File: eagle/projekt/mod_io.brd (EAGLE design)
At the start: 102.5 x 80 mm, 47 parts, among them IC1 PCF8574P

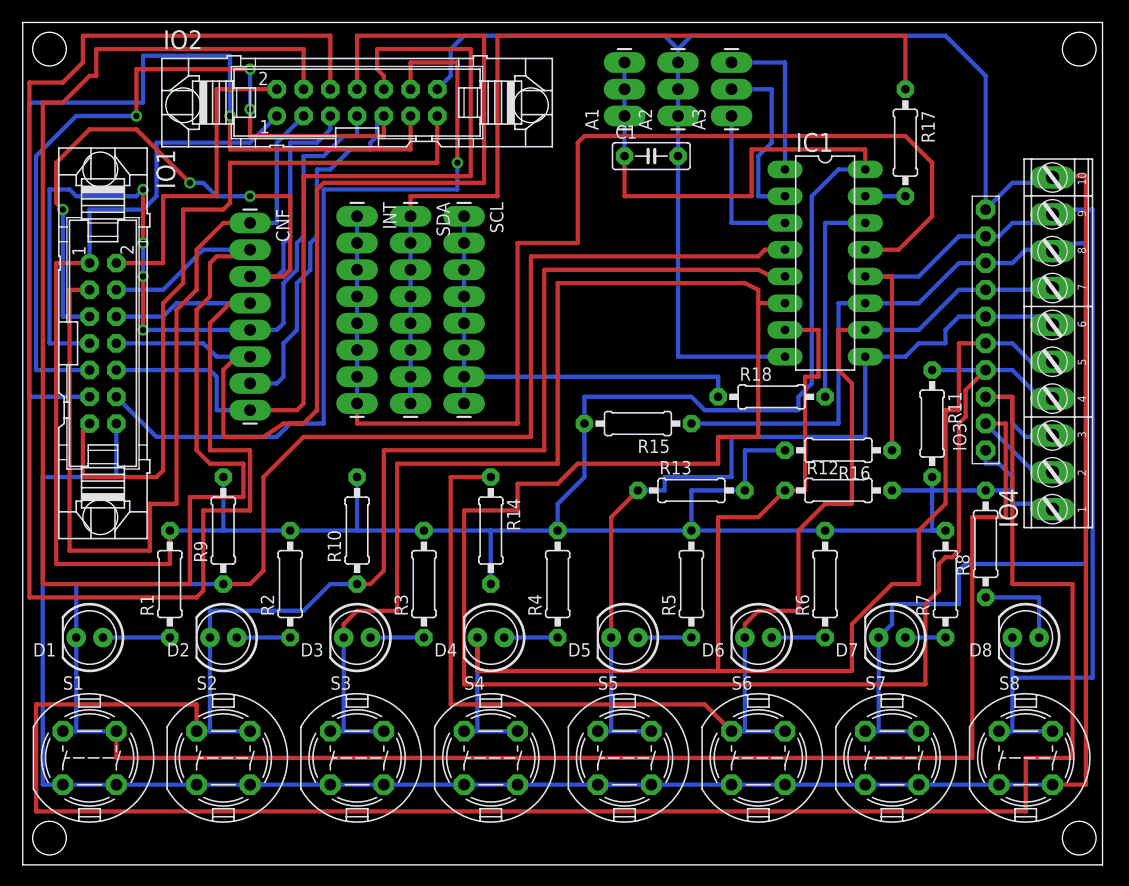
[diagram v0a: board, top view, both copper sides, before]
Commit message: Deska, modul IO
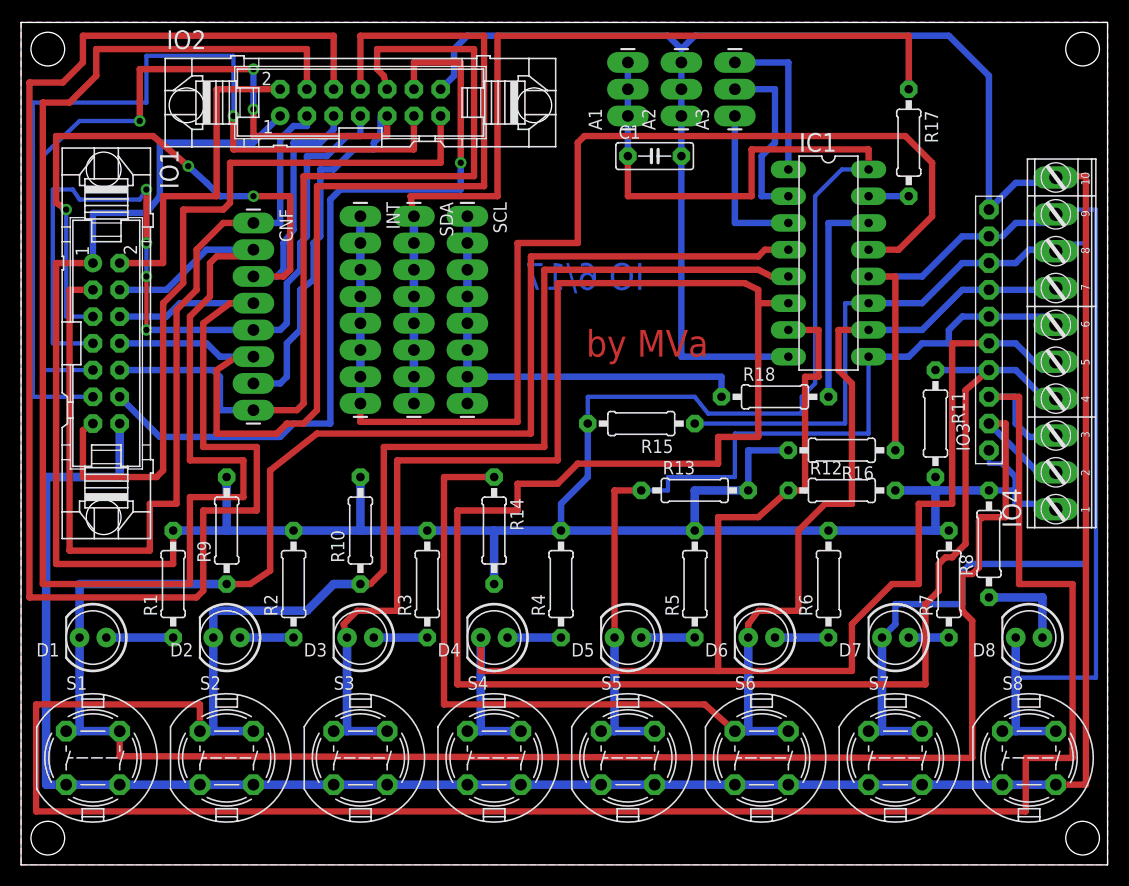
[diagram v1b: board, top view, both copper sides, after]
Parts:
- moved D6 0.32 mm to (70.2, 21.6)
- moved D7 0.32 mm to (82.9, 21.6)
- moved R17 0.32 mm to (84.1, 68.6)
- moved R7 0.32 mm to (87.9, 26.7)
- moved S6 0.32 mm to (70.2, 10.2)
- moved S7 0.32 mm to (82.9, 10.2)
- moved A1 0.32 mm to (57.5, 71.1)
- moved A2 0.32 mm to (62.5, 71.1)
- moved C1 0.32 mm to (60.0, 67.3)
- moved D3 0.32 mm to (32.1, 21.6)
- moved D5 0.32 mm to (57.5, 21.6)
- moved INT 0.32 mm to (32.1, 61.6)
- moved IO2 0.32 mm to (32.1, 72.4)
- moved R10 0.32 mm to (32.1, 31.8)
- moved R13 0.32 mm to (63.8, 35.6)
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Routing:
- net GPIO5: track 154.1 -> 157.2 mm
- net GPIO3: track 150.3 -> 152.5 mm
- net N$2: track 128.0 -> 129.9 mm
- net N$5: track 243.5 -> 245.3 mm
- net N$1: track 85.0 -> 86.5 mm
- net GPIO1: track 86.1 -> 87.5 mm
- net GPIO13: track 100.7 -> 101.8 mm
- net VCC: track 312.8 -> 313.9 mm
- net N$6: track 145.4 -> 146.5 mm
- net N$17: track 116.9 -> 116.0 mm
- net N$7: track 122.6 -> 122.0 mm
- net VIN: track 71.4 -> 72.0 mm
- net ADC: track 75.8 -> 75.2 mm
- added copper zone on layer 1, net N$24
- added copper zone on layer 16, net N$26
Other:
- board size 102.5 x 80 mm -> 103.2 x 80 mm
- board text added: "IO 6/17"
- board text added: "by MVa"
